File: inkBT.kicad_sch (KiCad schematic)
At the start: 4 parts, among them J1 AudioJack2_Ground, U1 LM2596S-3.3, U2 ESP32-WROOM-32, U3 PCM5102A

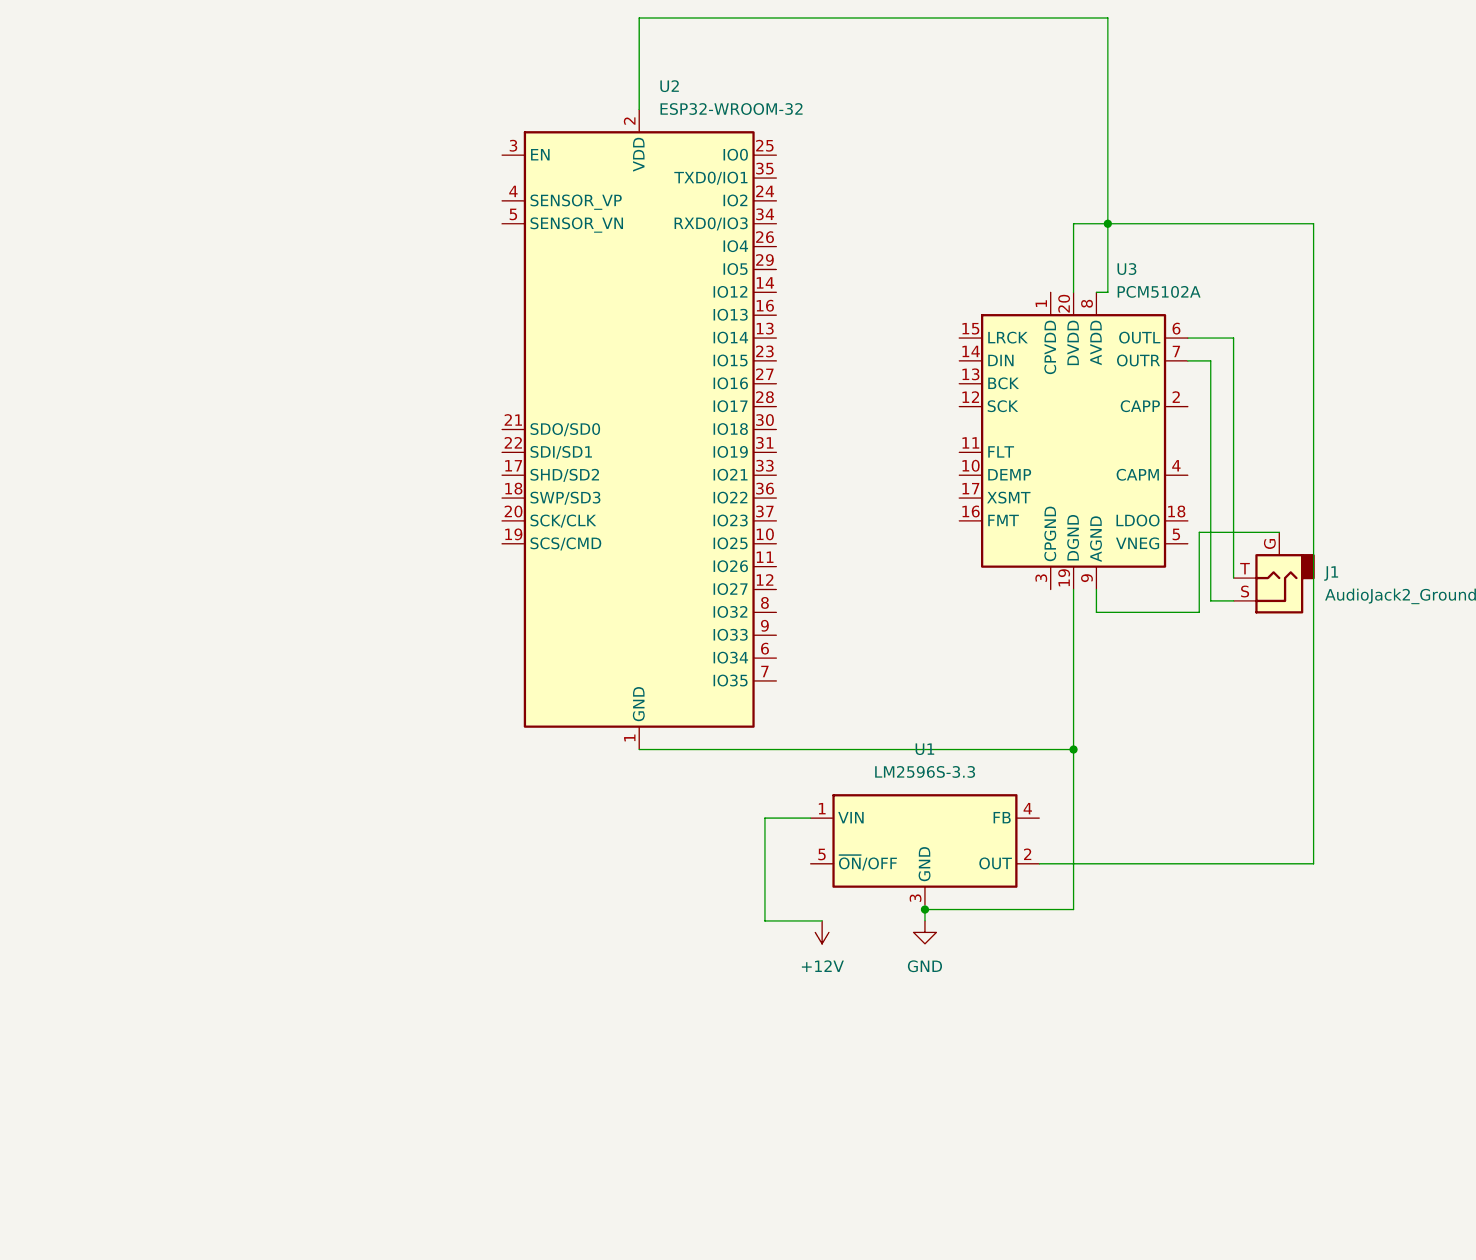
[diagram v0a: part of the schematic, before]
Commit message: a
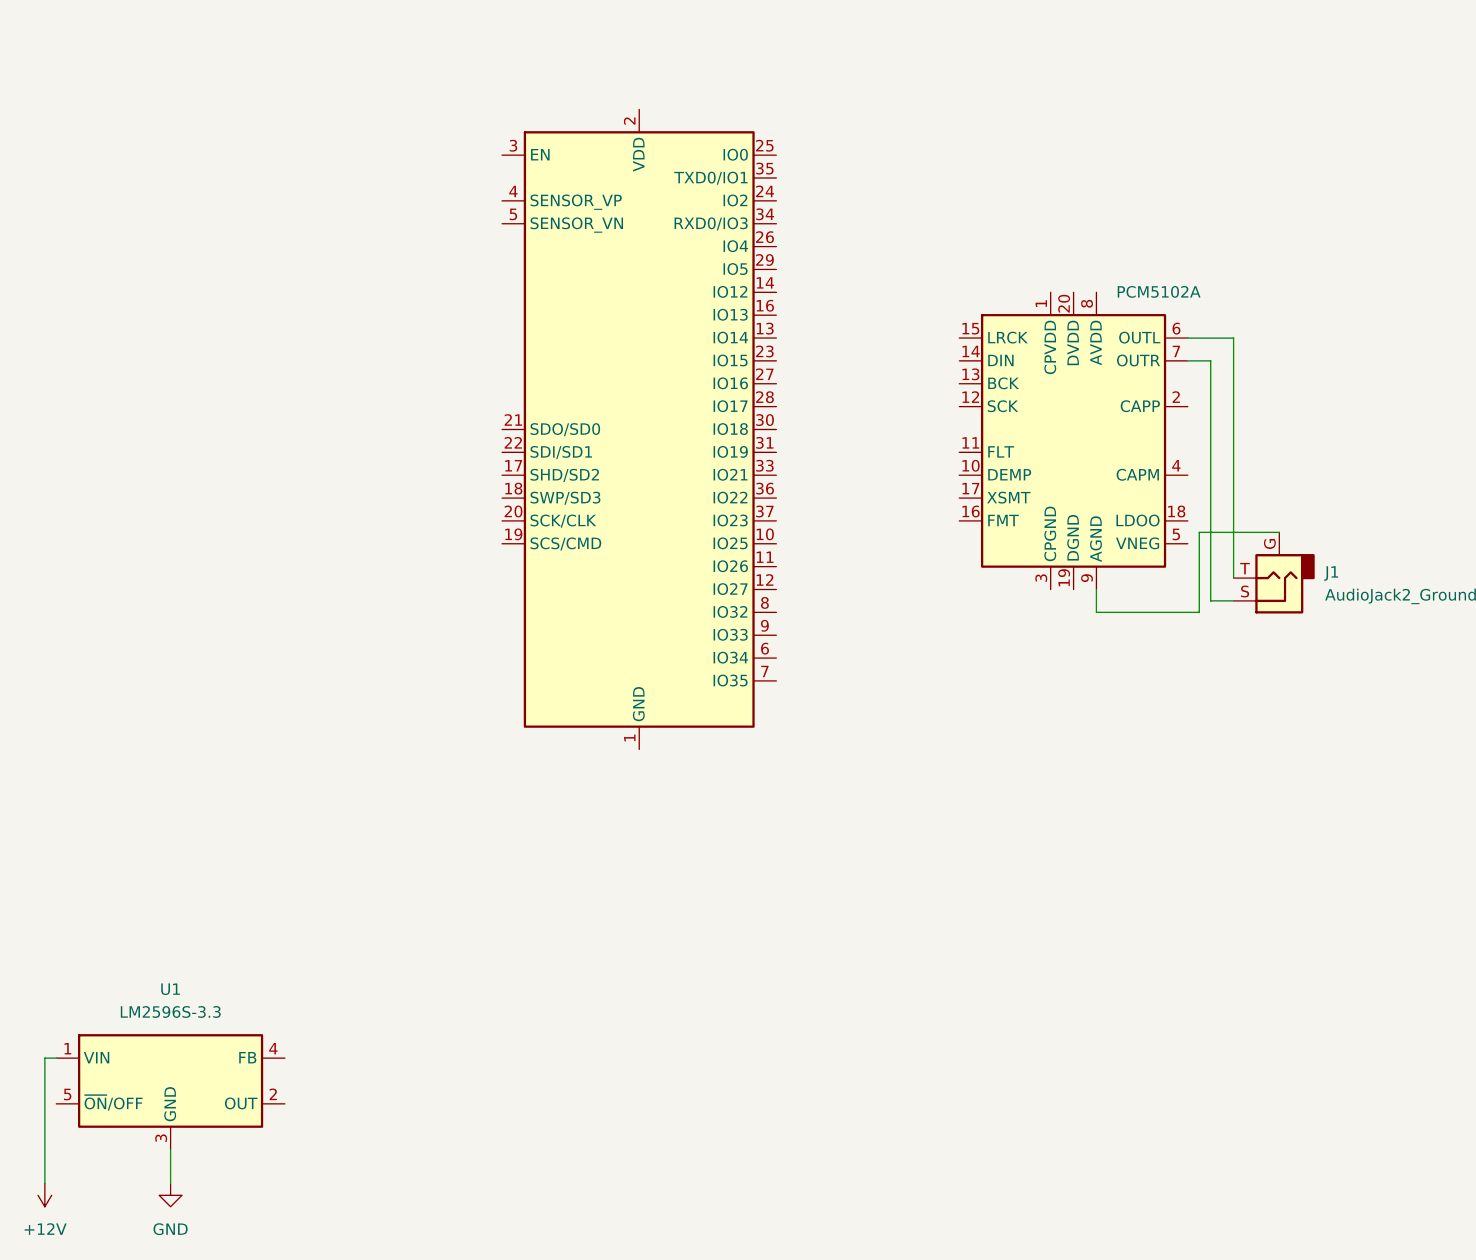
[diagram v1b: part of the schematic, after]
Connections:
- net GND: no longer U2.1 (GND), U2.15 (GND), U2.38 (GND), U2.39 (GND), U3.19 (DGND)
- new net: U2.1 (GND), U2.15 (GND), U2.38 (GND), U2.39 (GND)
- now unconnected: U1.2 (OUT), U2.2 (VDD), U3.20 (DVDD), U3.8 (AVDD)
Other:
- moved on the sheet: U1
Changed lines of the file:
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@@
 	(generator_version "10.0")
 	(paper "A4")
-	(junction
-		(at 245.11 142.24)
-		(diameter 0)
-		(color 0 0 0 0)
-	)
-	(junction
-		(at 248.92 83.82)
-		(diameter 0)
-		(color 0 0 0 0)
-	)
-	(junction
-		(at 228.6 160.02)
-		(diameter 0)
-		(color 0 0 0 0)
-	)
-	(wire
-		(pts
-			(xy 196.85 71.12) (xy 196.85 60.96)
-		)
-		(stroke
-			(width 0)
-			(type default)
-		)
-	)
-	(wire
-		(pts
-			(xy 196.85 60.96) (xy 248.92 60.96)
-		)
-		(stroke
-			(width 0)
-			(type default)
-		)
-	)
-	(wire
-		(pts
-			(xy 248.92 83.82) (xy 248.92 91.44)
-		)
-		(stroke
-			(width 0)
-			(type default)
-		)
-	)
 	(wire
 		(pts
@@
 	(wire
 		(pts
-			(xy 271.78 154.94) (xy 271.78 83.82)
-		)
-		(stroke
-			(width 0)
-			(type default)
-		)
-	)
-	(wire
-		(pts
-			(xy 245.11 124.46) (xy 245.11 142.24)
-		)
-		(stroke
-			(width 0)
-			(type default)
-		)
-	)
-	(wire
-		(pts
-			(xy 217.17 161.29) (xy 210.82 161.29)
-		)
-		(stroke
-			(width 0)
-			(type default)
-		)
-	)
-	(wire
-		(pts
-			(xy 245.11 160.02) (xy 228.6 160.02)
-		)
-		(stroke
-			(width 0)
-			(type default)
-		)
-	)
-	(wire
-		(pts
 			(xy 247.65 127) (xy 247.65 124.46)
 		)
@@
 	(wire
 		(pts
-			(xy 248.92 91.44) (xy 247.65 91.44)
-		)
-		(stroke
-			(width 0)
-			(type default)
-		)
-	)
-	(wire
-		(pts
-			(xy 241.3 154.94) (xy 271.78 154.94)
-		)
-		(stroke
-			(width 0)
-			(type default)
-		)
-	)
-	(wire
-		(pts
-			(xy 210.82 149.86) (xy 215.9 149.86)
-		)
-		(stroke
-			(width 0)
-			(type default)
-		)
-	)
-	(wire
-		(pts
-			(xy 245.11 142.24) (xy 245.11 160.02)
-		)
-		(stroke
-			(width 0)
-			(type default)
-		)
-	)
-	(wire
-		(pts
-			(xy 210.82 161.29) (xy 210.82 149.86)
+			(xy 130.81 176.53) (xy 132.08 176.53)
 		)
 		(stroke
@@
 	(wire
 		(pts
-			(xy 245.11 83.82) (xy 245.11 91.44)
-		)
-		(stroke
-			(width 0)
-			(type default)
-		)
-	)
-	(wire
-		(pts
-			(xy 248.92 83.82) (xy 245.11 83.82)
+			(xy 130.81 190.5) (xy 130.81 176.53)
 		)
 		(stroke
@@
 	(wire
 		(pts
-			(xy 271.78 83.82) (xy 248.92 83.82)
-		)
-		(stroke
-			(width 0)
-			(type default)
-		)
-	)
-	(wire
-		(pts
-			(xy 248.92 60.96) (xy 248.92 83.82)
-		)
-		(stroke
-			(width 0)
-			(type default)
-		)
-	)
-	(wire
-		(pts
 			(xy 259.08 118.11) (xy 267.97 118.11)
 		)
@@
 	(wire
 		(pts
-			(xy 228.6 160.02) (xy 228.6 161.29)
+			(xy 144.78 186.69) (xy 144.78 190.5)
 		)
 		(stroke
@@
 		(pts
 			(xy 260.35 99.06) (xy 257.81 99.06)
-		)
-		(stroke
-			(width 0)
-			(type default)
-		)
-	)
-	(wire
-		(pts
-			(xy 196.85 142.24) (xy 245.11 142.24)
 		)
 		(stroke
@@
 	(symbol
 		(lib_id "power:+12V")
-		(at 217.17 161.29 180)
+		(at 130.81 190.5 180)
 		(unit 1)
 		(body_style 1)
@@
 		(fields_autoplaced yes)
 		(property "Reference" "#PWR02"
-			(at 217.17 157.48 0)
+			(at 130.81 186.69 0)
 			(hide yes)
 			(show_name no)
@@
 		)
 		(property "Value" "+12V"
-			(at 217.17 166.37 0)
+			(at 130.81 195.58 0)
 			(show_name no)
 			(do_not_autoplace no)
@@
 		)
 		(property "Footprint" ""
-			(at 217.17 161.29 0)
+			(at 130.81 190.5 0)
 			(hide yes)
 			(show_name no)
@@
 		)
 		(property "Datasheet" ""
-			(at 217.17 161.29 0)
+			(at 130.81 190.5 0)
 			(hide yes)
 			(show_name no)
@@
 		)
 		(property "Description" ""
-			(at 217.17 161.29 0)
+			(at 130.81 190.5 0)
 			(show_name no)
 			(do_not_autoplace no)
@@
 	(symbol
 		(lib_id "Regulator_Switching:LM2596S-3.3")
-		(at 228.6 152.4 0)
+		(at 144.78 179.07 0)
 		(unit 1)
 		(body_style 1)
@@
 		(fields_autoplaced yes)
 		(property "Reference" "U1"
-			(at 228.6 142.24 0)
+			(at 144.78 168.91 0)
 			(show_name no)
 			(do_not_autoplace no)
@@
 		)
 		(property "Value" "LM2596S-3.3"
-			(at 228.6 144.78 0)
+			(at 144.78 171.45 0)
 			(show_name no)
 			(do_not_autoplace no)
@@
 		)
 		(property "Footprint" "Package_TO_SOT_SMD:TO-263-5_TabPin3"
-			(at 229.87 158.75 0)
+			(at 146.05 185.42 0)
 			(hide yes)
 			(show_name no)
@@
 		)
 		(property "Datasheet" "http://www.ti.com/lit/ds/symlink/lm2596.pdf"
-			(at 228.6 152.4 0)
+			(at 144.78 179.07 0)
 			(hide yes)
 			(show_name no)
@@
 		)
 		(property "Description" ""
-			(at 228.6 152.4 0)
+			(at 144.78 179.07 0)
 			(show_name no)
 			(do_not_autoplace no)
@@
 		(property "Reference" "U3"
 			(at 249.8441 88.9 0)
+			(hide yes)
 			(show_name no)
 			(do_not_autoplace no)
@@
 	(symbol
 		(lib_id "power:GND")
-		(at 228.6 161.29 0)
+		(at 144.78 190.5 0)
 		(unit 1)
 		(body_style 1)
@@
 		(fields_autoplaced yes)
 		(property "Reference" "#PWR01"
-			(at 228.6 167.64 0)
+			(at 144.78 196.85 0)
 			(hide yes)
 			(show_name no)
@@
 		)
 		(property "Value" "GND"
-			(at 228.6 166.37 0)
+			(at 144.78 195.58 0)
 			(show_name no)
 			(do_not_autoplace no)
@@
 		)
 		(property "Footprint" ""
-			(at 228.6 161.29 0)
+			(at 144.78 190.5 0)
 			(hide yes)
 			(show_name no)
@@
 		)
 		(property "Datasheet" ""
-			(at 228.6 161.29 0)
+			(at 144.78 190.5 0)
 			(hide yes)
 			(show_name no)
@@
 		)
 		(property "Description" ""
-			(at 228.6 161.29 0)
+			(at 144.78 190.5 0)
 			(show_name no)
 			(do_not_autoplace no)
@@
 		(property "Reference" "U2"
 			(at 199.0441 68.58 0)
+			(hide yes)
 			(show_name no)
 			(do_not_autoplace no)
@@
 		(property "Value" "ESP32-WROOM-32"
 			(at 199.0441 71.12 0)
-			(show_name no)
-			(do_not_autoplace no)
+			(hide yes)
+			(show_name no)
+			(do_not_autoplace no)

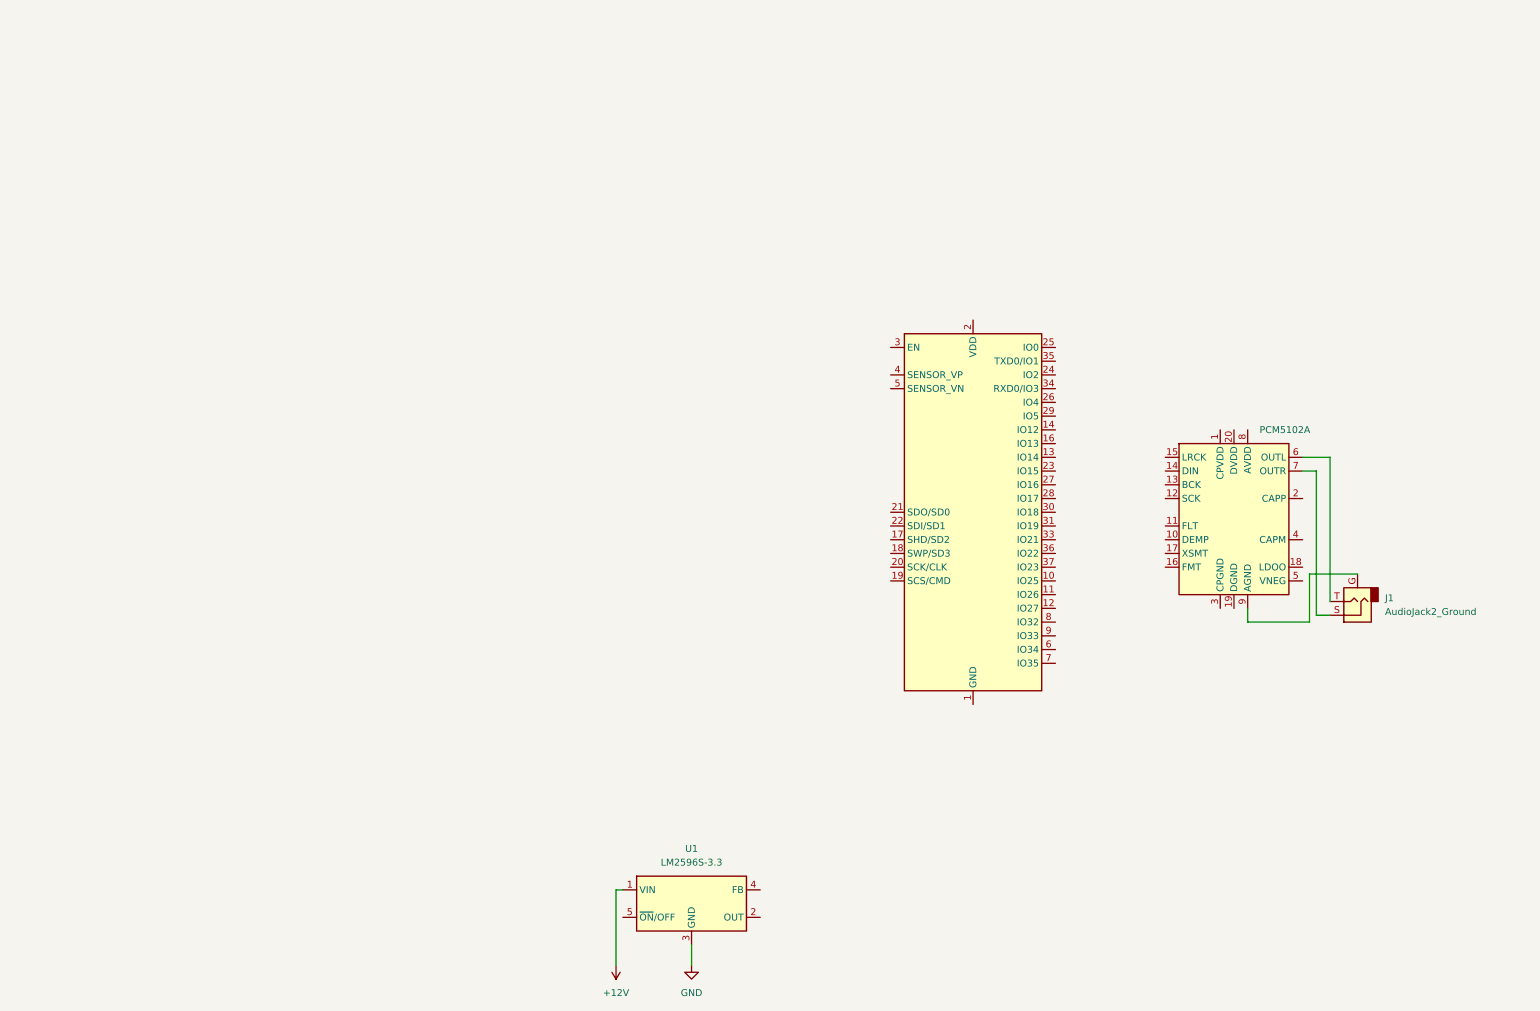
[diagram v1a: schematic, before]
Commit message: a
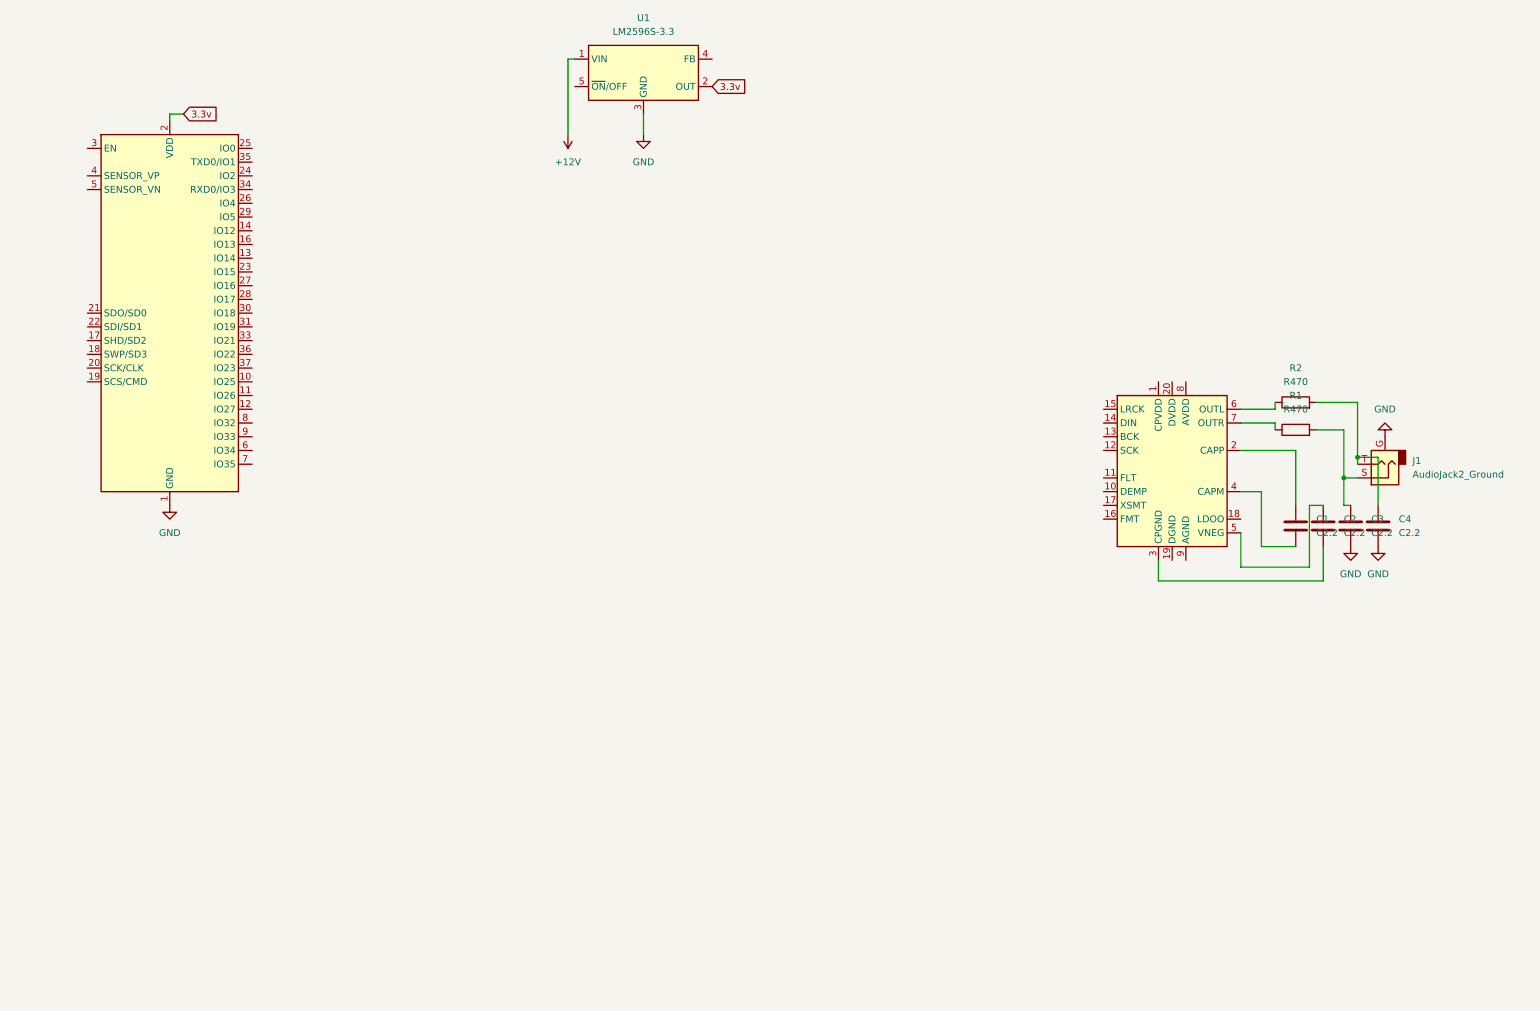
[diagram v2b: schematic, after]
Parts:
- added C1, C2, C3, C4: C2.2, Package_SO:SOIC-8_3.9x4.9mm_P1.27mm, symbol Device:C
- added R1, R2: R470, symbol Device:R
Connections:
- net GND: now also J1.G, U2.1 (GND), U2.15 (GND), U2.38 (GND), U2.39 (GND), C3.2, C4.2
- net 3.3v: now reaches U1.2 (OUT)
- net 3.3v: now also U2.2 (VDD)
- net at U3.2 (CAPP): now also C1.1
- net at U3.3 (CPGND): now also C2.2
- net at U3.4 (CAPM): now also C1.2
- net at U3.5 (VNEG): now also C2.1
- net at U3.6 (OUTL): now also R2.1; no longer J1.T
- net at U3.7 (OUTR): now also R1.1; no longer J1.S
- net at U3.9 (AGND): no longer J1.G
- new net: C3.1, J1.S, R1.2
- new net: C4.1, J1.T, R2.2
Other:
- moved on the sheet: J1, U1
